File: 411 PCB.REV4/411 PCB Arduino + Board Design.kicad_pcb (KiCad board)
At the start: 2 copper layers, 55 x 60 mm, 37 parts, among them J1 ICSP CONN, J3 Conn_01x04, J4 Conn_01x05_Pin, Q1 Q_NMOS_GDS, SW1 SW_SPST, SW2 SW_MEC_5E, SW3 SW_SPDT, SW4 SW_DPST_x2, U2 ATmega328P-P, Y1 8 MHz

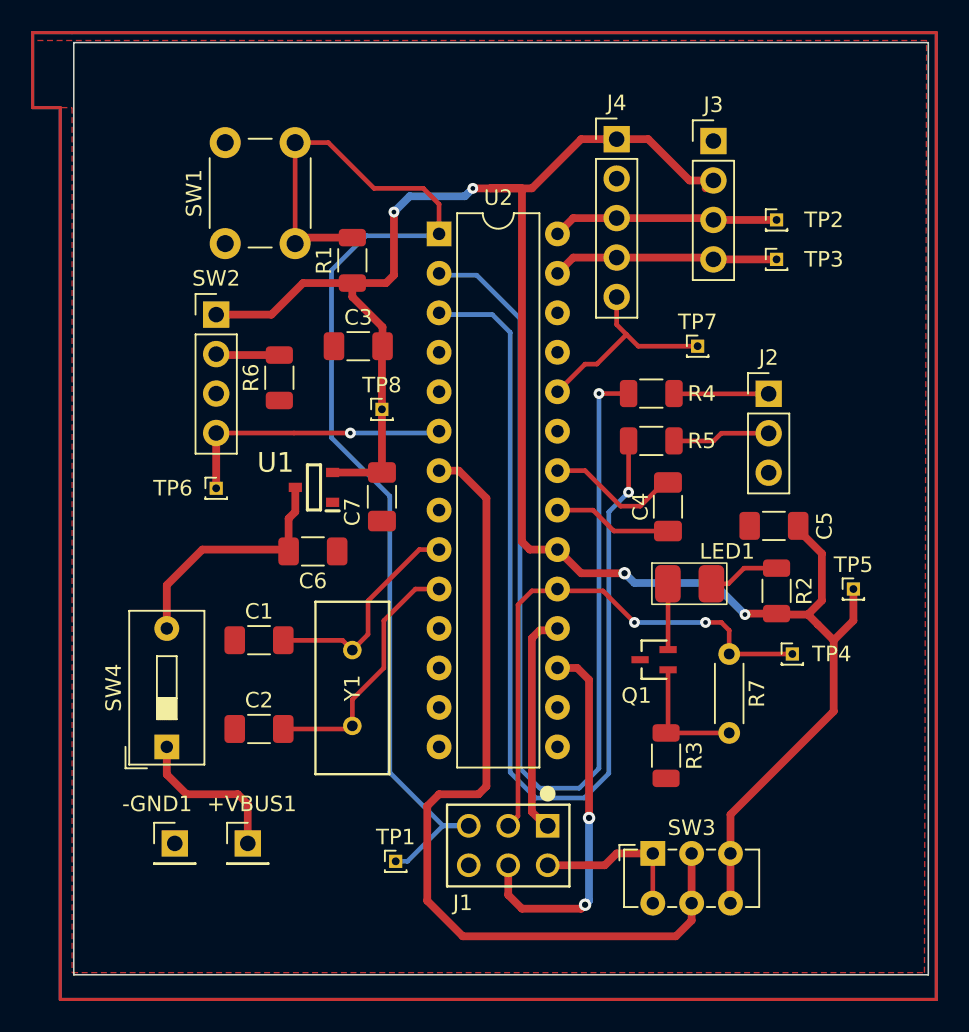
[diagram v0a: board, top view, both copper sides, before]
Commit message: Updated Board + PCB purchase receipt
Yes
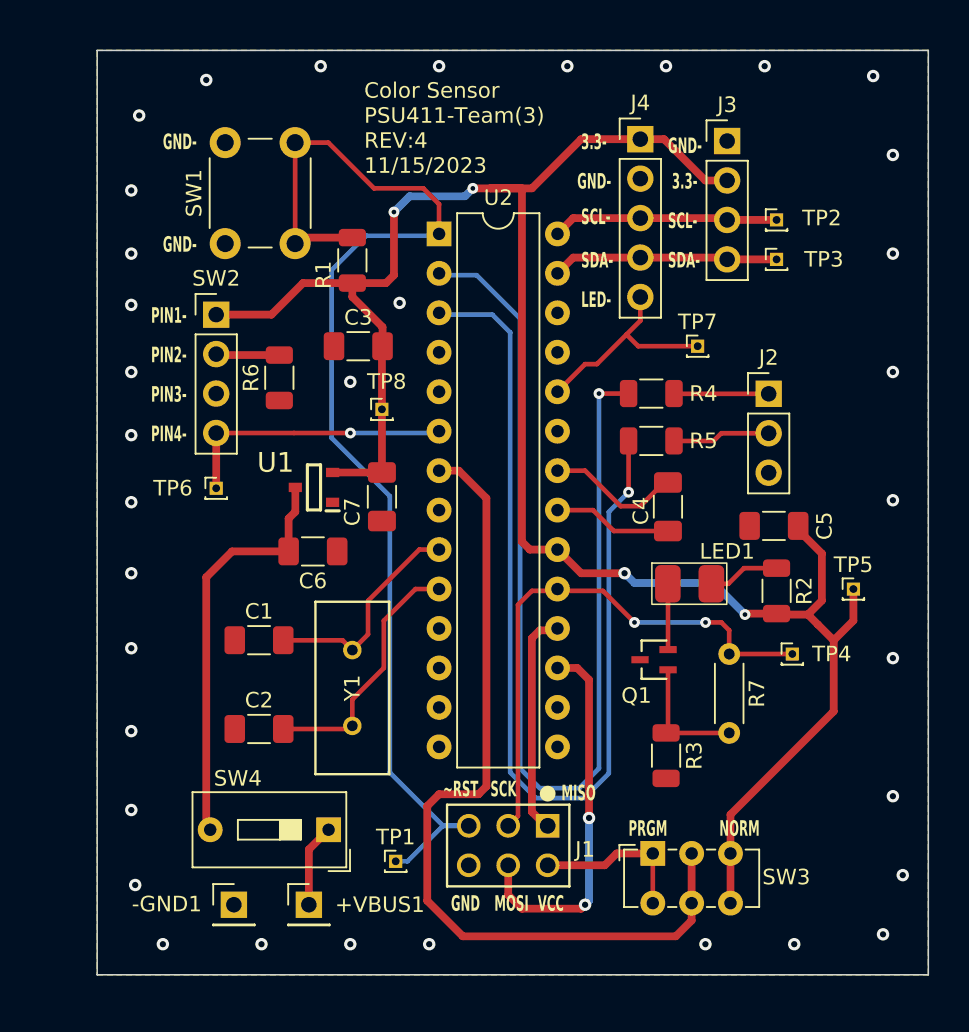
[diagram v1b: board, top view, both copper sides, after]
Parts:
- moved SW4 11.7 mm to (136.4, 105.7), turned to 180 degrees
- moved +VBUS1 5.57 mm to (135.1, 110.5)
- moved -GND1 5.48 mm to (130.3, 110.5)
- moved J4 1.52 mm to (156.5, 61.2)
- moved J3 0.88 mm to (162.1, 61.3)
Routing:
- net Net-(SW4A-B): track 15.9 -> 26.6 mm
- net Net-(+VBUS1-Pin_1): track 10.3 -> 5.35 mm
- net GND: vias 0 -> 35
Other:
- board size 55 x 60 mm -> 53.5 x 59.5 mm
- board text added: "3.3-"
- board text added: "Color Sensor PSU411-Team(3) REV:4 11/15/2023"
- board text added: "GND"
- board text added: "GND-"
- board text added: "LED-"
- board text added: "MISO"
- board text added: "MOSI"
- board text added: "NORM"
- board text added: "PIN1-"
- board text added: "PIN2-"
- board text added: "PIN3-"
- board text added: "PIN4-"
- board text added: "PRGM"
- board text added: "SCK"
- board text added: "SCL-"
- board text added: "SDA-"
- board text added: "VCC"
- board text added: "~RST"
